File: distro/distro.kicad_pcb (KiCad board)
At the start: 2 copper layers, 59.1 x 76.8 mm, 20 parts, among them K1 CONN_3, K2 CONN_3, K3 CONN_3, K4 CONN_3, P4 CONN_2, P5 CONN_2, P6 CONN_2, P7 CONN_2, P8 CONN_2

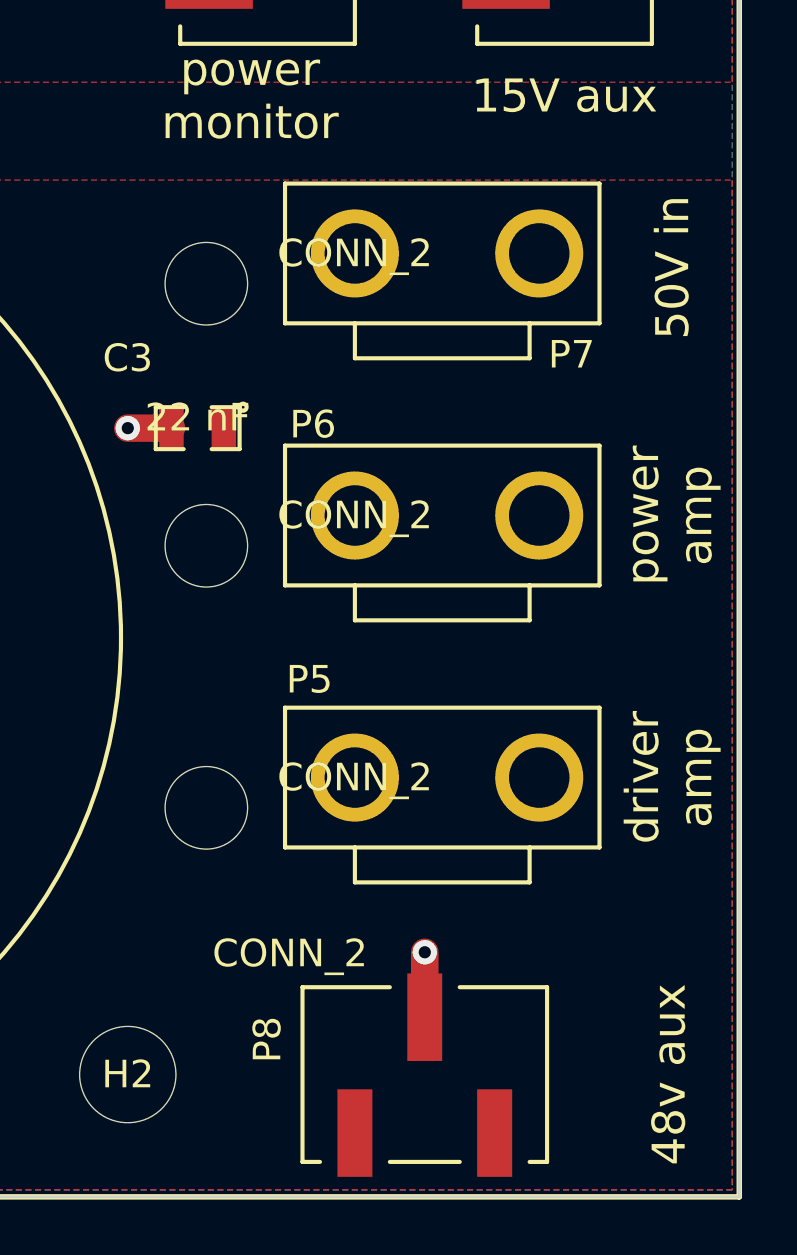
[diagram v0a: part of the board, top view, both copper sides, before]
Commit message: DFM changes after last protoype rev
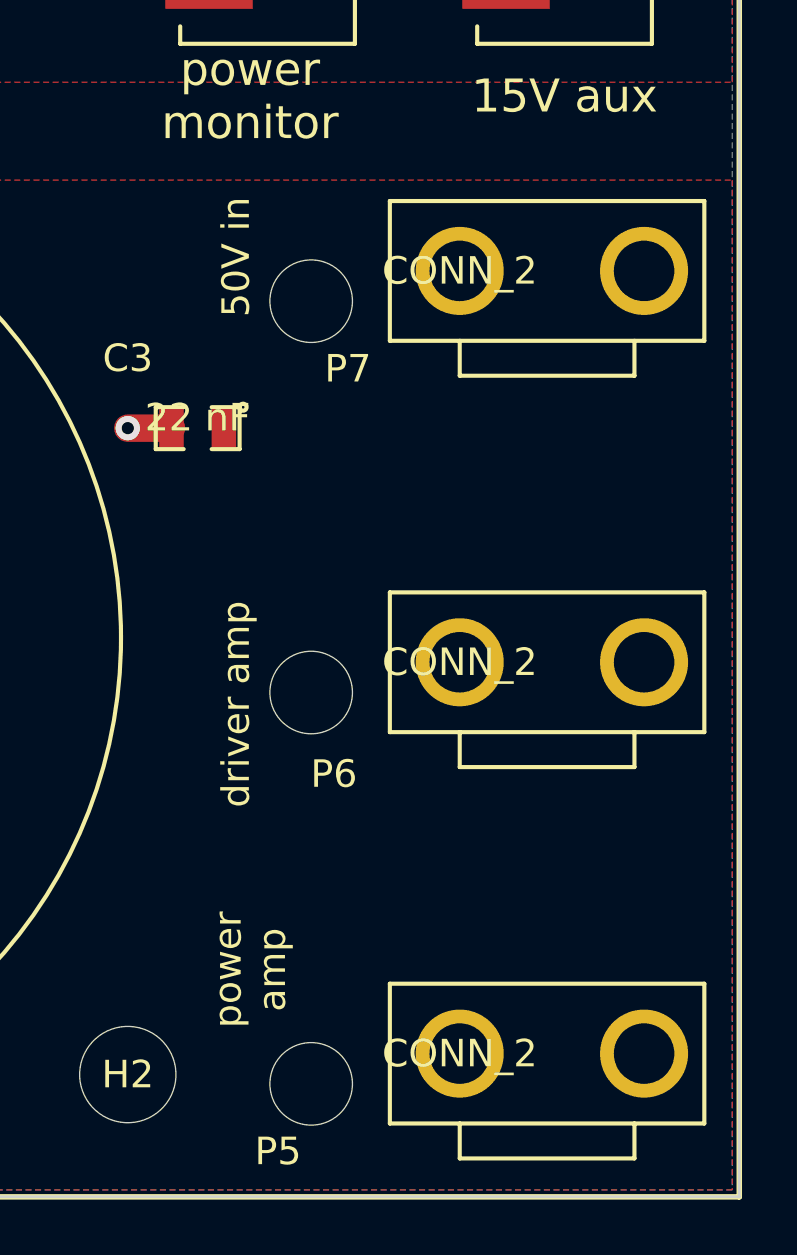
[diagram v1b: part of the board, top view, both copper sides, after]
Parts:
- removed P8: CONN_2, sdtransmitter:0740991003
- moved P5 10.7 mm to (125.7, 133.5)
- moved P6 6.55 mm to (125.7, 119.3)
- moved P7 3.86 mm to (125.7, 105.1)
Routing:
- net GND: track 24.7 -> 22.3 mm, vias 10 -> 9
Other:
- board text removed: "48v aux"
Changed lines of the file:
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@@
 (kicad_pcb (version 3) (host pcbnew "(2014-03-19 BZR 4756)-product")
   (general
-    (links 26)
+    (links 24)
     (no_connects 0)
-    (area 74.829572 61.812499 137.247572 140.38276)
+    (area 76.784999 61.862499 135.940001 138.797501)
     (thickness 1.6)
-    (drawings 19)
-    (tracks 20)
+    (drawings 18)
+    (tracks 18)
     (zones 0)
-    (modules 20)
+    (modules 19)
     (nets 4)
   )
@@
   )
   (module local:0015311026 (layer F.Cu)
-    (at 121.92 113.9825 180)
-    (fp_text reference P6 (at 1.524 3.302 180) (layer F.SilkS)
+    (at 125.73 119.3165 180)
+    (fp_text reference P6 (at 4.572 -4.064 180) (layer F.SilkS)
       (effects (font (size 1 1) (thickness 0.25)))
     )
@@
   )
   (module local:0015311026 (layer F.Cu)
-    (at 121.92 104.4575 180)
-    (fp_text reference P7 (at -7.874 -3.683 360) (layer F.SilkS)
+    (at 125.73 105.0925 180)
+    (fp_text reference P7 (at 4.064 -3.556 360) (layer F.SilkS)
       (effects (font (size 1 1) (thickness 0.25)))
     )
@@
     (pad "" np_thru_hole circle (at 5.4 -1.1 180) (size 3 3) (drill 3) (layers *.Cu *.Mask F.SilkS))
   )
-  (module sdtransmitter:0740991003 (layer F.Cu)
-    (at 124.46 134.3025)
-    (fp_text reference P8 (at -5.715 -1.27 90) (layer F.SilkS)
-      (effects (font (size 1 1) (thickness 0.25)))
-    )
-    (fp_text value CONN_2 (at -4.9 -4.4) (layer F.SilkS)
-      (effects (font (size 1 1) (thickness 0.25)))
-    )
-    (fp_line (start -1.27 3.175) (end 1.27 3.175) (layer F.SilkS) (width 0.15))
-    (fp_line (start -4.445 -3.175) (end -1.27 -3.175) (layer F.SilkS) (width 0.15))
-    (fp_line (start -3.81 3.175) (end -4.445 3.175) (layer F.SilkS) (width 0.15))
-    (fp_line (start -4.445 3.175) (end -4.445 -3.175) (layer F.SilkS) (width 0.15))
-    (fp_line (start 1.27 -3.175) (end 4.445 -3.175) (layer F.SilkS) (width 0.15))
-    (fp_line (start 4.445 -3.175) (end 4.445 3.175) (layer F.SilkS) (width 0.15))
-    (fp_line (start 4.445 3.175) (end 3.81 3.175) (layer F.SilkS) (width 0.15))
-    (pad 1 smd rect (at -2.54 2.127) (size 1.27 3.18) (layers F.Cu F.Paste F.Mask)
-      (net 3 VCC))
-    (pad 2 smd rect (at 0 -2.083) (size 1.27 3.18) (layers F.Cu F.Paste F.Mask)
-      (net 2 GND))
-    (pad 3 smd rect (at 2.54 2.127) (size 1.27 3.18) (layers F.Cu F.Paste F.Mask))
-  )
   (module Mounting_Holes:MountingHole_3-5mm (layer F.Cu)
     (at 81.28 66.3575)
@@
   )
   (module local:0015311026 (layer F.Cu)
-    (at 121.92 123.5075 180)
-    (fp_text reference P5 (at 1.651 3.556 180) (layer F.SilkS)
+    (at 125.73 133.5405 180)
+    (fp_text reference P5 (at 6.604 -3.556 180) (layer F.SilkS)
       (effects (font (size 1 1) (thickness 0.25)))
     )
@@
     (effects (font (size 1.5 1.5) (thickness 0.3)) (justify mirror))
   )
-  (gr_text "50V in" (at 133.477 104.9655 90) (layer F.SilkS)
-    (effects (font (size 1.2 1.2) (thickness 0.3)))
-  )
-  (gr_text "driver\namp" (at 133.35 123.5075 90) (layer F.SilkS)
-    (effects (font (size 1.2 1.2) (thickness 0.3)))
-  )
-  (gr_text "power\namp" (at 133.35 113.9825 90) (layer F.SilkS)
-    (effects (font (size 1.2 1.2) (thickness 0.3)))
+  (gr_text "50V in" (at 117.602 104.5845 90) (layer F.SilkS)
+    (effects (font (size 1 1) (thickness 0.25)))
+  )
+  (gr_text "driver amp" (at 117.602 120.8405 90) (layer F.SilkS)
+    (effects (font (size 1 1) (thickness 0.25)))
+  )
+  (gr_text "power\namp" (at 118.11 130.4925 90) (layer F.SilkS)
+    (effects (font (size 1 1) (thickness 0.25)))
   )
   (gr_text "15V in" (at 132.08 70.8025) (layer F.SilkS)
@@
     (effects (font (size 1.2 1.2) (thickness 0.3)))
   )
-  (gr_text "48v aux" (at 133.35 134.3025 90) (layer F.SilkS)
-    (effects (font (size 1.2 1.2) (thickness 0.3)))
-  )
+  (via (at 113.665 110.8075) (size 0.889) (layers F.Cu B.Cu) (net 2))
+  (segment (start 115.2525 110.8075) (end 113.665 110.8075) (width 1) (layer F.Cu) (net 2))
+  (via (at 121.92 73.3425) (size 0.889) (layers F.Cu B.Cu) (net 2))
+  (segment (start 123.5075 73.3425) (end 121.92 73.3425) (width 1) (layer F.Cu) (net 2))
+  (via (at 119.38 77.1525) (size 0.889) (layers F.Cu B.Cu) (net 2))
+  (segment (start 116.618 77.1525) (end 119.38 77.1525) (width 1) (layer F.Cu) (net 2))
+  (via (at 118.11 79.6925) (size 0.889) (layers F.Cu B.Cu) (net 2))
+  (segment (start 120.828 79.6925) (end 118.11 79.6925) (width 1) (layer F.Cu) (net 2))
+  (via (at 128.905 79.6925) (size 0.889) (layers F.Cu B.Cu) (net 2))
+  (segment (start 131.623 79.6925) (end 128.905 79.6925) (width 1) (layer F.Cu) (net 2))
+  (via (at 119.38 89.8525) (size 0.889) (layers F.Cu B.Cu) (net 2))
+  (segment (start 116.618 89.8525) (end 119.38 89.8525) (width 1) (layer F.Cu) (net 2))
+  (via (at 118.11 92.3925) (size 0.889) (layers F.Cu B.Cu) (net 2))
+  (segment (start 120.828 92.3925) (end 118.11 92.3925) (width 1) (layer F.Cu) (net 2))
+  (via (at 130.175 89.8525) (size 0.889) (layers F.Cu B.Cu) (net 2))
+  (segment (start 127.413 89.8525) (end 130.175 89.8525) (width 1) (layer F.Cu) (net 2))
+  (via (at 128.905 92.3925) (size 0.889) (layers F.Cu B.Cu) (net 2))
   (segment (start 131.623 92.3925) (end 128.905 92.3925) (width 1) (layer F.Cu) (net 2))
-  (via (at 128.905 92.3925) (size 0.889) (layers F.Cu B.Cu) (net 2))
-  (segment (start 127.413 89.8525) (end 130.175 89.8525) (width 1) (layer F.Cu) (net 2))
-  (via (at 130.175 89.8525) (size 0.889) (layers F.Cu B.Cu) (net 2))
-  (segment (start 120.828 92.3925) (end 118.11 92.3925) (width 1) (layer F.Cu) (net 2))
-  (via (at 118.11 92.3925) (size 0.889) (layers F.Cu B.Cu) (net 2))
-  (segment (start 116.618 89.8525) (end 119.38 89.8525) (width 1) (layer F.Cu) (net 2))
-  (via (at 119.38 89.8525) (size 0.889) (layers F.Cu B.Cu) (net 2))
-  (segment (start 131.623 79.6925) (end 128.905 79.6925) (width 1) (layer F.Cu) (net 2))
-  (via (at 128.905 79.6925) (size 0.889) (layers F.Cu B.Cu) (net 2))
-  (segment (start 120.828 79.6925) (end 118.11 79.6925) (width 1) (layer F.Cu) (net 2))
-  (via (at 118.11 79.6925) (size 0.889) (layers F.Cu B.Cu) (net 2))
-  (segment (start 116.618 77.1525) (end 119.38 77.1525) (width 1) (layer F.Cu) (net 2))
-  (via (at 119.38 77.1525) (size 0.889) (layers F.Cu B.Cu) (net 2))
-  (segment (start 123.5075 73.3425) (end 121.92 73.3425) (width 1) (layer F.Cu) (net 2))
-  (via (at 121.92 73.3425) (size 0.889) (layers F.Cu B.Cu) (net 2))
-  (segment (start 124.46 132.2195) (end 124.46 129.8575) (width 1) (layer F.Cu) (net 2))
-  (via (at 124.46 129.8575) (size 0.889) (layers F.Cu B.Cu) (net 2))
-  (segment (start 115.2525 110.8075) (end 113.665 110.8075) (width 1) (layer F.Cu) (net 2))
-  (via (at 113.665 110.8075) (size 0.889) (layers F.Cu B.Cu) (net 2))
   (zone (net 2) (net_name GND) (layer B.Cu) (hatch edge 0.508)
     (connect_pads (clearance 0.5))
